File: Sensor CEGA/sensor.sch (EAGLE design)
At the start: 8 parts, among them J1 22-27-2021-02, J2 22-27-2031-03

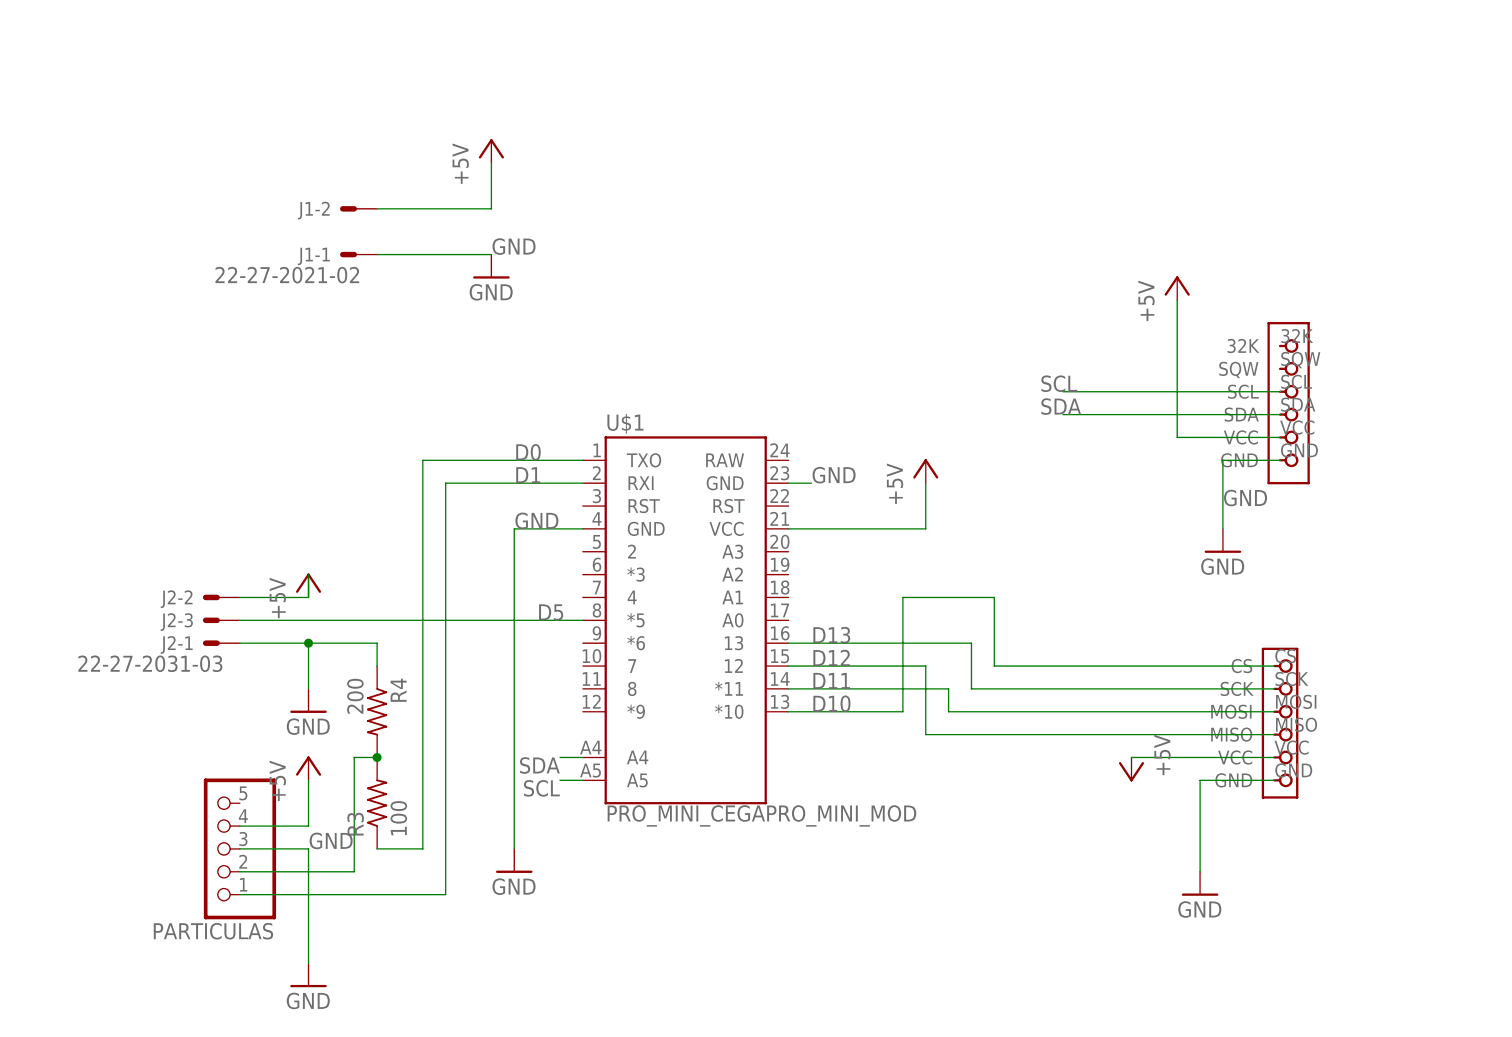
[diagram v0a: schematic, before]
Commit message: add libraries
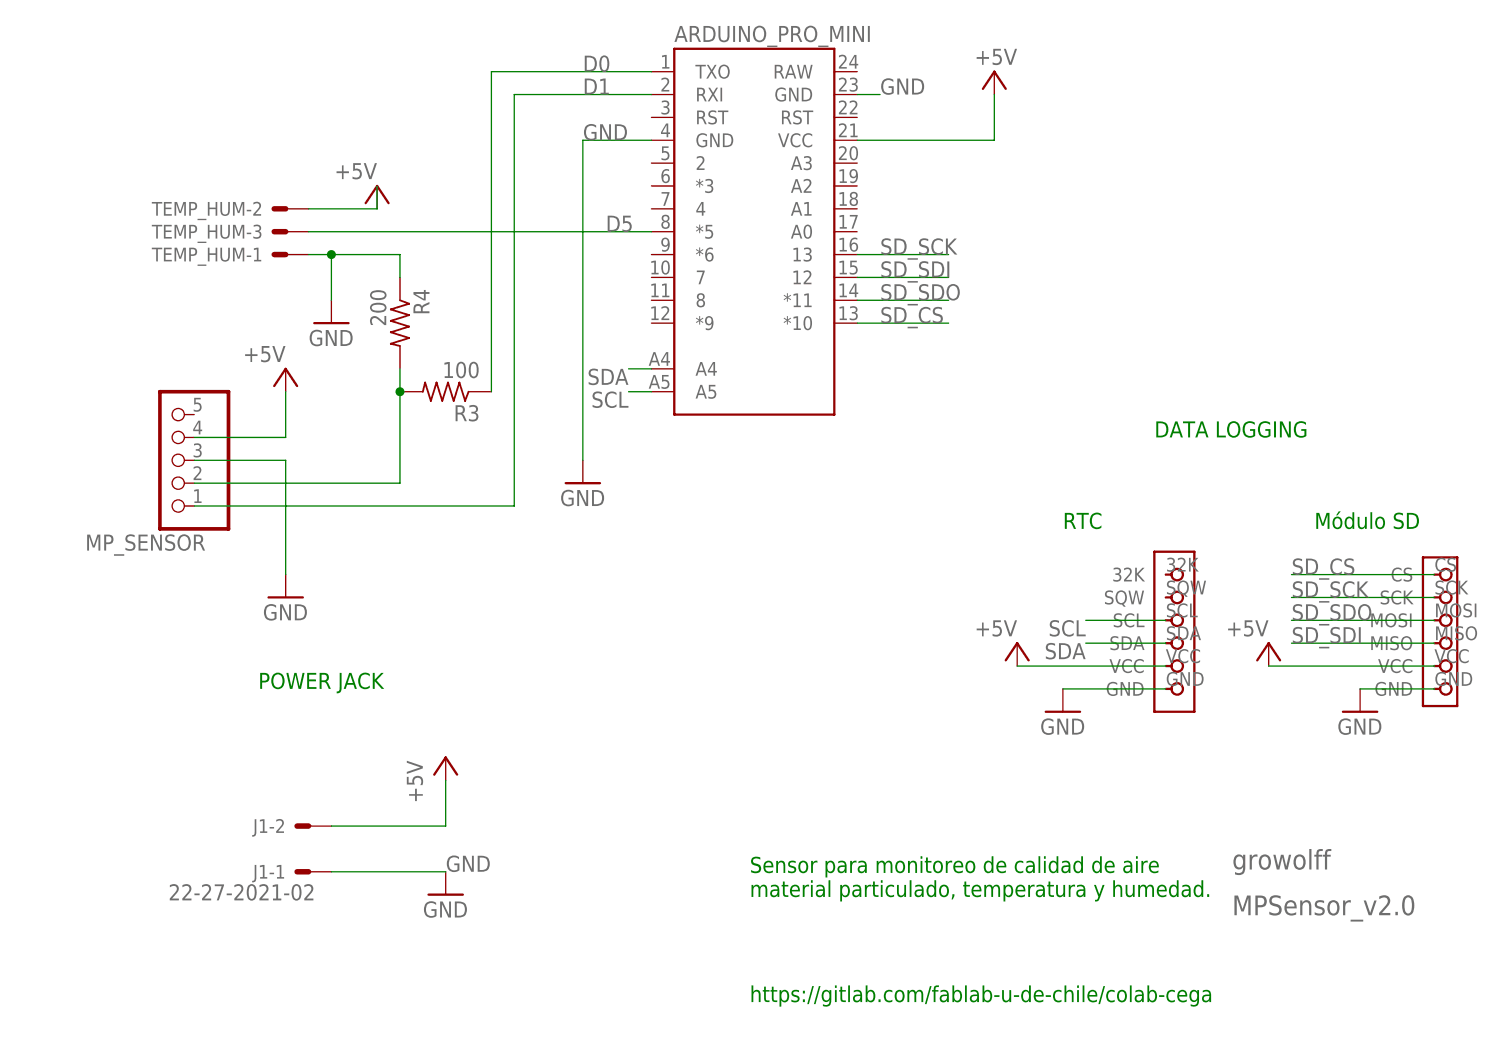
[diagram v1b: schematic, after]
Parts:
- removed J2: 22-27-2031-03, con-molex:22-27-2031-03
- removed PARTICULAS: (no value), pinhead:PINHD-1X5
- removed U$1: PRO_MINI_CEGAPRO_MINI_MOD, fablab_uchile:PRO_MINI_CEGAPRO_MINI_MOD
- added ARDUINO_PRO_MINI: PRO_MINI_CEGAPRO_MINI_MOD, fablab_uchile:PRO_MINI_CEGAPRO_MINI_MOD
- added MP_SENSOR: (no value), pinhead:PINHD-1X5
- added TEMP_HUM: 22-27-2031-03, con-molex:22-27-2031-03
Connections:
- removed net D10: SD_READER.CS, U$1.*10
- removed net D11: SD_READER.MOSI, U$1.*11
- removed net D12: SD_READER.MISO, U$1.12
- removed net D13: SD_READER.SCK, U$1.13
- new net SD_CS: ARDUINO_PRO_MINI.*10, SD_READER.CS
- new net SD_SCK: ARDUINO_PRO_MINI.13, SD_READER.SCK
- new net SD_SDI: ARDUINO_PRO_MINI.12, SD_READER.MISO
- new net SD_SDO: ARDUINO_PRO_MINI.*11, SD_READER.MOSI
- net +5V: now also ARDUINO_PRO_MINI.VCC, MP_SENSOR.4, TEMP_HUM-2.S; no longer J2-2.S, PARTICULAS.4, U$1.VCC
- net D0: now also ARDUINO_PRO_MINI.TXO; no longer U$1.TXO
- net D1: now also ARDUINO_PRO_MINI.RXI, MP_SENSOR.1; no longer PARTICULAS.1, U$1.RXI
- net D5: now also ARDUINO_PRO_MINI.*5, TEMP_HUM-3.S; no longer J2-3.S, U$1.*5
- net GND: now also ARDUINO_PRO_MINI.GND, ARDUINO_PRO_MINI.GND@2, MP_SENSOR.3, TEMP_HUM-1.S; no longer J2-1.S, PARTICULAS.3, U$1.GND, U$1.GND@2
- net N$2: now also MP_SENSOR.2; no longer PARTICULAS.2
- net SCL: now also ARDUINO_PRO_MINI.A5; no longer U$1.A5
- net SDA: now also ARDUINO_PRO_MINI.A4; no longer U$1.A4
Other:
- note added: "DATA LOGGING"
- note added: "MPSensor_v2.0"
- note added: "Módulo SD"
- note added: "POWER JACK"
- note added: "RTC"
- note added: "Sensor para monitoreo de calidad de aire material particulado, temperatura y humedad."
- note added: "growolff"
- note added: "https://gitlab.com/fablab-u-de-chile/colab-cega"
- moved on the sheet: J1-1, J1-2, R3, R4
